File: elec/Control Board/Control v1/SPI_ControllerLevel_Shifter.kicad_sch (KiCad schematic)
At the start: 0 parts

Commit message: Add Lees PublicInvention submodule library. Update Control V1 project and schematic for new library.
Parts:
- added C301, C302, C303, C304: 39PF, Capacitor_SMD:C_0603_1608Metric_Pad1.08x0.95mm_HandSolder, symbol Device:C
- added C305, C306: 1uF, Capacitor_SMD:C_0603_1608Metric_Pad1.08x0.95mm_HandSolder, symbol Device:C
- added J301: RJ12_6P6C_HORZ, PubInv_PCB:RJ12_Amphenol_54601, symbol GPAD_SCH_LIB:RJ12_6P6C_HORZ
- added J302: 0.100_2Pin, Connector_PinHeader_2.54mm:PinHeader_1x02_P2.54mm_Vertical, symbol GPAD_SCH_LIB:22-23-2021
- added Q301, Q302, Q303, Q304: BSS138, Package_TO_SOT_SMD:SOT-23, symbol Transistor_FET:BSS138
- added R301, R302, R311: 1R, Resistor_SMD:R_0603_1608Metric_Pad0.98x0.95mm_HandSolder, symbol Device:R
- added R303, R304, R305, R307, R312, R315: DNI, Resistor_SMD:R_0603_1608Metric_Pad0.98x0.95mm_HandSolder, symbol Device:R
- added R306, R309, R310, R314: 1K, Resistor_SMD:R_0603_1608Metric_Pad0.98x0.95mm_HandSolder, symbol Device:R
- added R308, R313, R316, R317: 10K, Resistor_SMD:R_0603_1608Metric_Pad0.98x0.95mm_HandSolder, symbol Device:R
- added TP301: ControllerVCC, TestPoint:TestPoint_Loop_D2.54mm_Drill1.5mm_Beaded, symbol Connector:TestPoint
- added TP302: CPIO, TestPoint:TestPoint_Loop_D2.54mm_Drill1.5mm_Beaded, symbol Connector:TestPoint
- added TP303: SCK, TestPoint:TestPoint_Loop_D2.54mm_Drill1.5mm_Beaded, symbol Connector:TestPoint
- added TP304: COPI, TestPoint:TestPoint_Loop_D2.54mm_Drill1.5mm_Beaded, symbol Connector:TestPoint
- added TP305: nCS, TestPoint:TestPoint_Loop_D2.54mm_Drill1.5mm_Beaded, symbol Connector:TestPoint
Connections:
- new net: R312.1, R315.2
- new net +12forSPIPeripherial: J302.2, R301.2
- new net +3V3LevelShift: R311.1
- new net +3V3Local: C305.1, Q301.1 (G), Q302.1 (G), Q303.1 (G), Q304.1 (G), R311.2, R313.1, R314.1, R316.1, R317.1
- new net +5LevelShift: R302.1
- new net +5VLocal: C306.1, R302.2, R306.1, R308.1, R309.1, R310.1
- new net CIPO: C301.1, J301.6, Q302.3 (D), R303.1, R308.2, TP302.1
- new net CIPO_3V3: Q302.2 (S), R303.2, R312.2, R314.2
- new net COPI: C303.1, J301.2, Q304.3 (D), R305.1, R310.2, TP304.1
- new net COPI_3V3: Q304.2 (S), R305.2, R317.2
- new net COPI_nCS: Q301.2 (S), R307.2, R313.2
- new net C_SCK: C302.1, J301.4, Q303.3 (D), R304.1, R309.2, TP303.1
- new net ControllerVcc: J301.5, J302.1, R301.1, TP301.1
- new net GND: C301.2, C302.2, C303.2, C304.2, C305.2, C306.2, J301.3, R315.1
- new net SCK_3V3: Q303.2 (S), R304.2, R316.2
- new net nCS: C304.1, J301.1, Q301.3 (D), R306.2, R307.1, TP305.1
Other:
- note added: "An RJ12 Connector for SPI with 5V logic level."
- note added: "An interface card for the COG to bring out SPI bus for the GPAD. Level shift from 5V to 3V on the CIPO."
- note added: "CIPO: Controller In, Peripherial Out C_SCK: Controller Serial Clock (output) COPI: Controler Out, Peripherial In nCS: not Chip Select, ie /CHIP_SELECT"
- note added: "SPI 3V3 to 5V Controller Interface"
- note added: "SPI Connector Signal Names"

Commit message: Add footrpint to Max31850 module.
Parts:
- J301: footprint PubInv_PCB:RJ12_Amphenol_54601 -> PubInv_KiCad_PCB:RJ12_Amphenol_54601
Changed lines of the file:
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@@
       (project "Control v1"
         (path "/c68c9deb-8d4d-42f0-adf8-4d3022f4ee59/1f0b18fc-1fda-489e-a08b-a0ece1be6922"
-          (reference "#PWR050") (unit 1)
+          (reference "#PWR047") (unit 1)
         )
       )
@@
       (project "Control v1"
         (path "/c68c9deb-8d4d-42f0-adf8-4d3022f4ee59/1f0b18fc-1fda-489e-a08b-a0ece1be6922"
-          (reference "R30") (unit 1)
+          (reference "R34") (unit 1)
         )
       )
@@
       (project "Control v1"
         (path "/c68c9deb-8d4d-42f0-adf8-4d3022f4ee59/1f0b18fc-1fda-489e-a08b-a0ece1be6922"
-          (reference "R32") (unit 1)
+          (reference "R36") (unit 1)
         )
       )
@@
       (project "Control v1"
         (path "/c68c9deb-8d4d-42f0-adf8-4d3022f4ee59/1f0b18fc-1fda-489e-a08b-a0ece1be6922"
-          (reference "R38") (unit 1)
+          (reference "R42") (unit 1)
         )
       )
@@
       (project "Control v1"
         (path "/c68c9deb-8d4d-42f0-adf8-4d3022f4ee59/1f0b18fc-1fda-489e-a08b-a0ece1be6922"
-          (reference "TP2") (unit 1)
+          (reference "TP3") (unit 1)
         )
       )
@@
       (project "Control v1"
         (path "/c68c9deb-8d4d-42f0-adf8-4d3022f4ee59/1f0b18fc-1fda-489e-a08b-a0ece1be6922"
-          (reference "#PWR049") (unit 1)
+          (reference "#PWR046") (unit 1)
         )
       )
@@
       (project "Control v1"
         (path "/c68c9deb-8d4d-42f0-adf8-4d3022f4ee59/1f0b18fc-1fda-489e-a08b-a0ece1be6922"
-          (reference "R27") (unit 1)
+          (reference "R31") (unit 1)
         )
       )
@@
       (project "Control v1"
         (path "/c68c9deb-8d4d-42f0-adf8-4d3022f4ee59/1f0b18fc-1fda-489e-a08b-a0ece1be6922"
-          (reference "R35") (unit 1)
+          (reference "R39") (unit 1)
         )
       )
@@
       (project "Control v1"
         (path "/c68c9deb-8d4d-42f0-adf8-4d3022f4ee59/1f0b18fc-1fda-489e-a08b-a0ece1be6922"
-          (reference "R40") (unit 1)
+          (reference "R44") (unit 1)
         )
       )
@@
       (project "Control v1"
         (path "/c68c9deb-8d4d-42f0-adf8-4d3022f4ee59/1f0b18fc-1fda-489e-a08b-a0ece1be6922"
-          (reference "R28") (unit 1)
+          (reference "R32") (unit 1)
         )
       )
@@
       (project "Control v1"
         (path "/c68c9deb-8d4d-42f0-adf8-4d3022f4ee59/1f0b18fc-1fda-489e-a08b-a0ece1be6922"
-          (reference "R36") (unit 1)
+          (reference "R40") (unit 1)
         )
       )
@@
       (project "Control v1"
         (path "/c68c9deb-8d4d-42f0-adf8-4d3022f4ee59/1f0b18fc-1fda-489e-a08b-a0ece1be6922"
-          (reference "R39") (unit 1)
+          (reference "R43") (unit 1)
         )
       )
@@
       (project "Control v1"
         (path "/c68c9deb-8d4d-42f0-adf8-4d3022f4ee59/1f0b18fc-1fda-489e-a08b-a0ece1be6922"
-          (reference "#PWR052") (unit 1)
+          (reference "#PWR049") (unit 1)
         )
       )
@@
       (project "Control v1"
         (path "/c68c9deb-8d4d-42f0-adf8-4d3022f4ee59/1f0b18fc-1fda-489e-a08b-a0ece1be6922"
-          (reference "R24") (unit 1)
+          (reference "R28") (unit 1)
         )
       )
@@
       (project "Control v1"
         (path "/c68c9deb-8d4d-42f0-adf8-4d3022f4ee59/1f0b18fc-1fda-489e-a08b-a0ece1be6922"
-          (reference "TP1") (unit 1)
+          (reference "TP2") (unit 1)
         )
       )
@@
       (project "Control v1"
         (path "/c68c9deb-8d4d-42f0-adf8-4d3022f4ee59/1f0b18fc-1fda-489e-a08b-a0ece1be6922"
-          (reference "TP4") (unit 1)
+          (reference "TP5") (unit 1)
         )
       )
@@
       (project "Control v1"
         (path "/c68c9deb-8d4d-42f0-adf8-4d3022f4ee59/1f0b18fc-1fda-489e-a08b-a0ece1be6922"
-          (reference "#PWR046") (unit 1)
+          (reference "#PWR043") (unit 1)
         )
       )
@@
       (project "Control v1"
         (path "/c68c9deb-8d4d-42f0-adf8-4d3022f4ee59/1f0b18fc-1fda-489e-a08b-a0ece1be6922"
-          (reference "R25") (unit 1)
+          (reference "R29") (unit 1)
         )
       )
@@
       (project "Control v1"
         (path "/c68c9deb-8d4d-42f0-adf8-4d3022f4ee59/1f0b18fc-1fda-489e-a08b-a0ece1be6922"
-          (reference "#PWR053") (unit 1)
+          (reference "#PWR050") (unit 1)
         )
       )
@@
       (project "Control v1"
         (path "/c68c9deb-8d4d-42f0-adf8-4d3022f4ee59/1f0b18fc-1fda-489e-a08b-a0ece1be6922"
-          (reference "#PWR051") (unit 1)
+          (reference "#PWR048") (unit 1)
         )
       )
@@
       (project "Control v1"
         (path "/c68c9deb-8d4d-42f0-adf8-4d3022f4ee59/1f0b18fc-1fda-489e-a08b-a0ece1be6922"
-          (reference "J23") (unit 1)
+          (reference "J20") (unit 1)
         )
       )
@@
       (project "Control v1"
         (path "/c68c9deb-8d4d-42f0-adf8-4d3022f4ee59/1f0b18fc-1fda-489e-a08b-a0ece1be6922"
-          (reference "TP5") (unit 1)
+          (reference "TP6") (unit 1)
         )
       )
@@
       (project "Control v1"
         (path "/c68c9deb-8d4d-42f0-adf8-4d3022f4ee59/1f0b18fc-1fda-489e-a08b-a0ece1be6922"
-          (reference "#PWR047") (unit 1)
+          (reference "#PWR044") (unit 1)
         )
       )
@@
       (project "Control v1"
         (path "/c68c9deb-8d4d-42f0-adf8-4d3022f4ee59/1f0b18fc-1fda-489e-a08b-a0ece1be6922"
-          (reference "R26") (unit 1)
+          (reference "R30") (unit 1)
         )
       )
@@
       (project "Control v1"
         (path "/c68c9deb-8d4d-42f0-adf8-4d3022f4ee59/1f0b18fc-1fda-489e-a08b-a0ece1be6922"
-          (reference "TP3") (unit 1)
+          (reference "TP4") (unit 1)
         )
       )
@@
       (project "Control v1"
         (path "/c68c9deb-8d4d-42f0-adf8-4d3022f4ee59/1f0b18fc-1fda-489e-a08b-a0ece1be6922"
-          (reference "#PWR048") (unit 1)
+          (reference "#PWR045") (unit 1)
         )
       )
@@
       (project "Control v1"
         (path "/c68c9deb-8d4d-42f0-adf8-4d3022f4ee59/1f0b18fc-1fda-489e-a08b-a0ece1be6922"
-          (reference "R29") (unit 1)
+          (reference "R33") (unit 1)
         )
       )
@@
       (project "Control v1"
         (path "/c68c9deb-8d4d-42f0-adf8-4d3022f4ee59/1f0b18fc-1fda-489e-a08b-a0ece1be6922"
-          (reference "R34") (unit 1)
+          (reference "R38") (unit 1)
         )
       )
@@
       (project "Control v1"
         (path "/c68c9deb-8d4d-42f0-adf8-4d3022f4ee59/1f0b18fc-1fda-489e-a08b-a0ece1be6922"
-          (reference "R31") (unit 1)
+          (reference "R35") (unit 1)
         )
       )
@@
       (effects (font (size 1.27 1.27)))
     )
-    (property "Footprint" "PubInv_PCB:RJ12_Amphenol_54601" (at 41.021 106.68 90)
+    (property "Footprint" "PubInv_KiCad_PCB:RJ12_Amphenol_54601" (at 41.021 106.68 90)
       (effects (font (size 1.27 1.27)) hide)
     )
@@
       (project "Control v1"
         (path "/c68c9deb-8d4d-42f0-adf8-4d3022f4ee59/1f0b18fc-1fda-489e-a08b-a0ece1be6922"
-          (reference "J22") (unit 1)
+          (reference "J19") (unit 1)
         )
       )
@@
       (project "Control v1"
         (path "/c68c9deb-8d4d-42f0-adf8-4d3022f4ee59/1f0b18fc-1fda-489e-a08b-a0ece1be6922"
-          (reference "R33") (unit 1)
+          (reference "R37") (unit 1)
         )
       )
@@
       (project "Control v1"
         (path "/c68c9deb-8d4d-42f0-adf8-4d3022f4ee59/1f0b18fc-1fda-489e-a08b-a0ece1be6922"
-          (reference "R37") (unit 1)
-        )
-      )
+          (reference "R41") (unit 1)
+        )
+      )

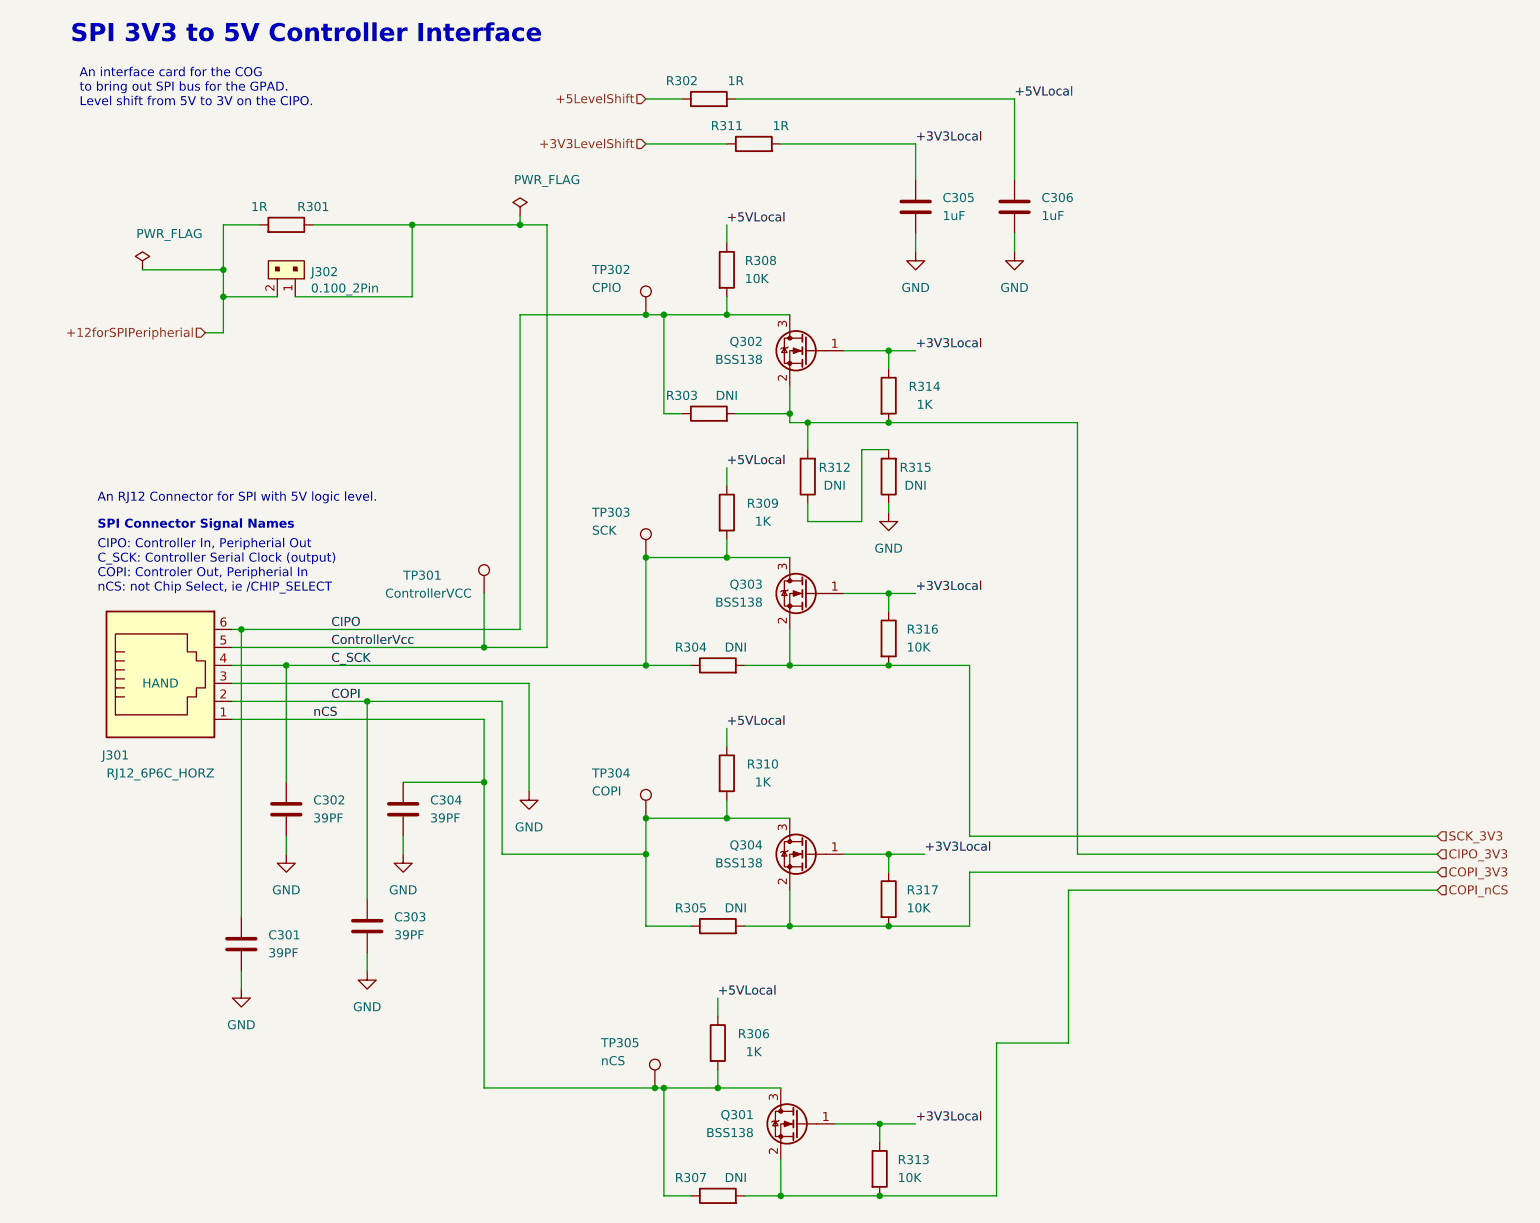
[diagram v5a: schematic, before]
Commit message: Fix swome ERC errors.
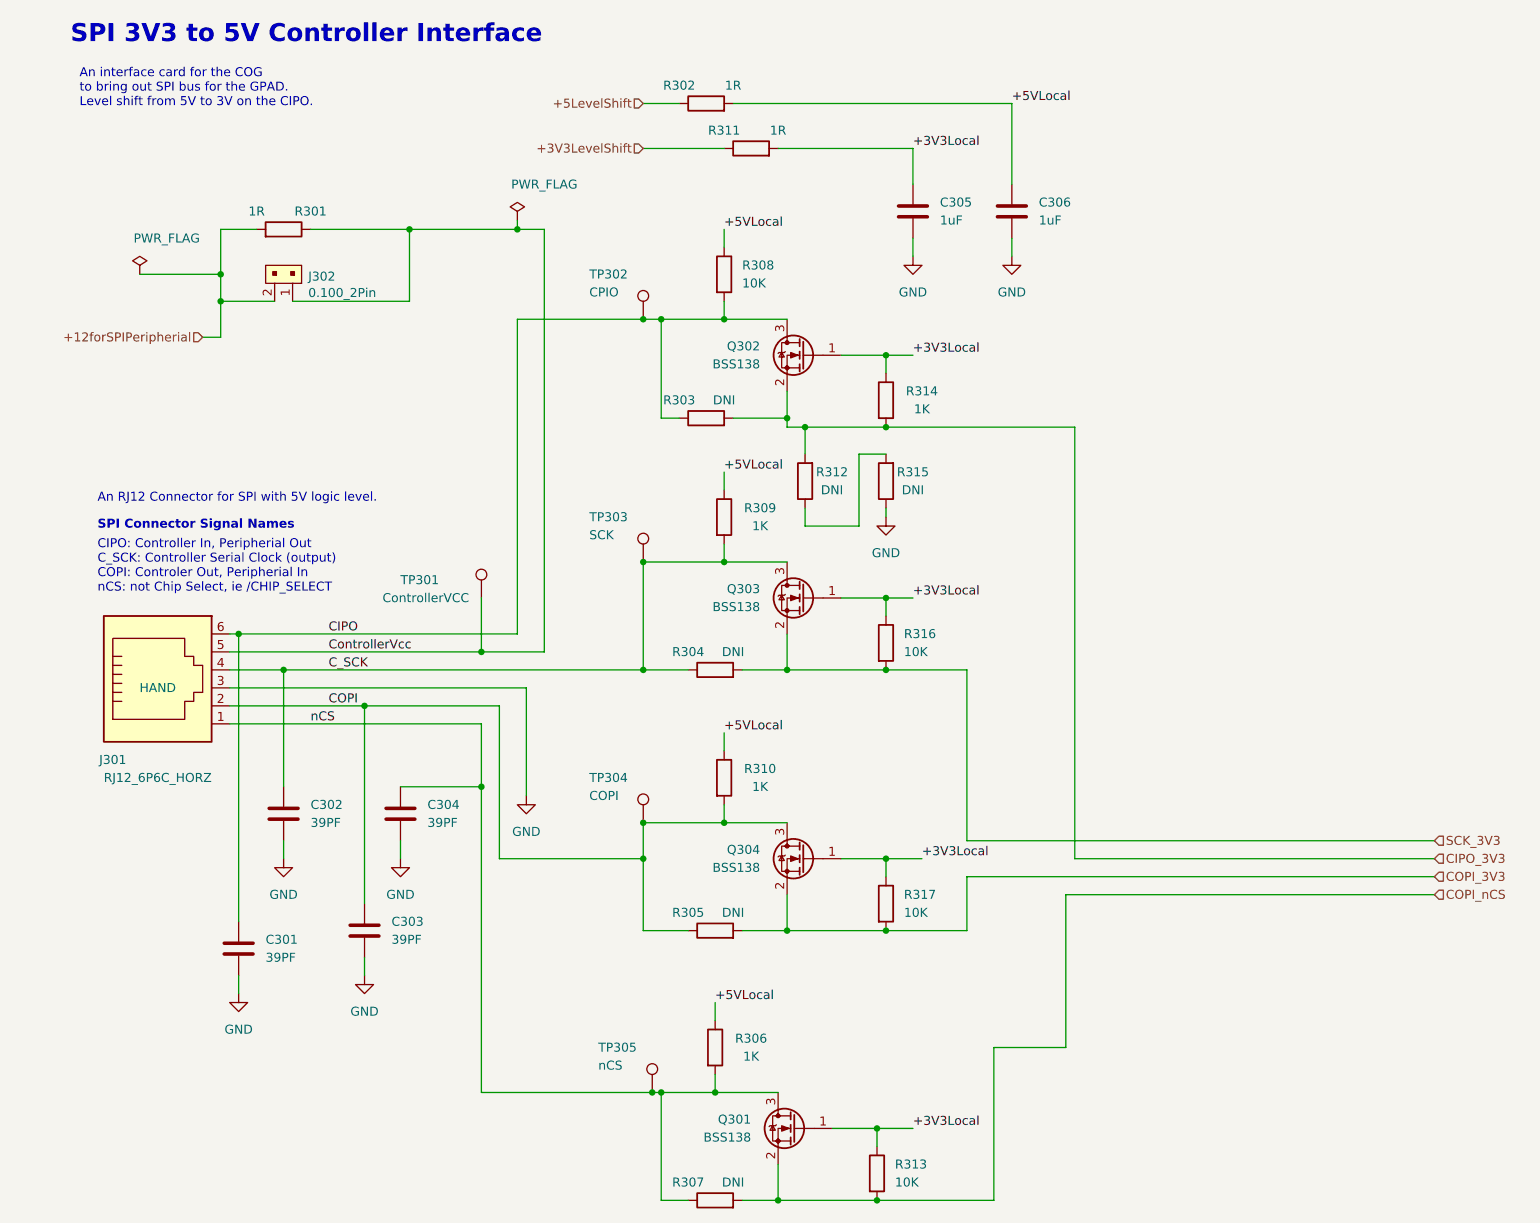
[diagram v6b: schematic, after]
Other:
- moved on the sheet: C301, C302, C303, C304, C305, C306, J301, J302, Q301, Q302, Q303, Q304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
